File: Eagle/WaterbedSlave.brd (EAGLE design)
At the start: 55.3 x 50.4 mm, 6 parts

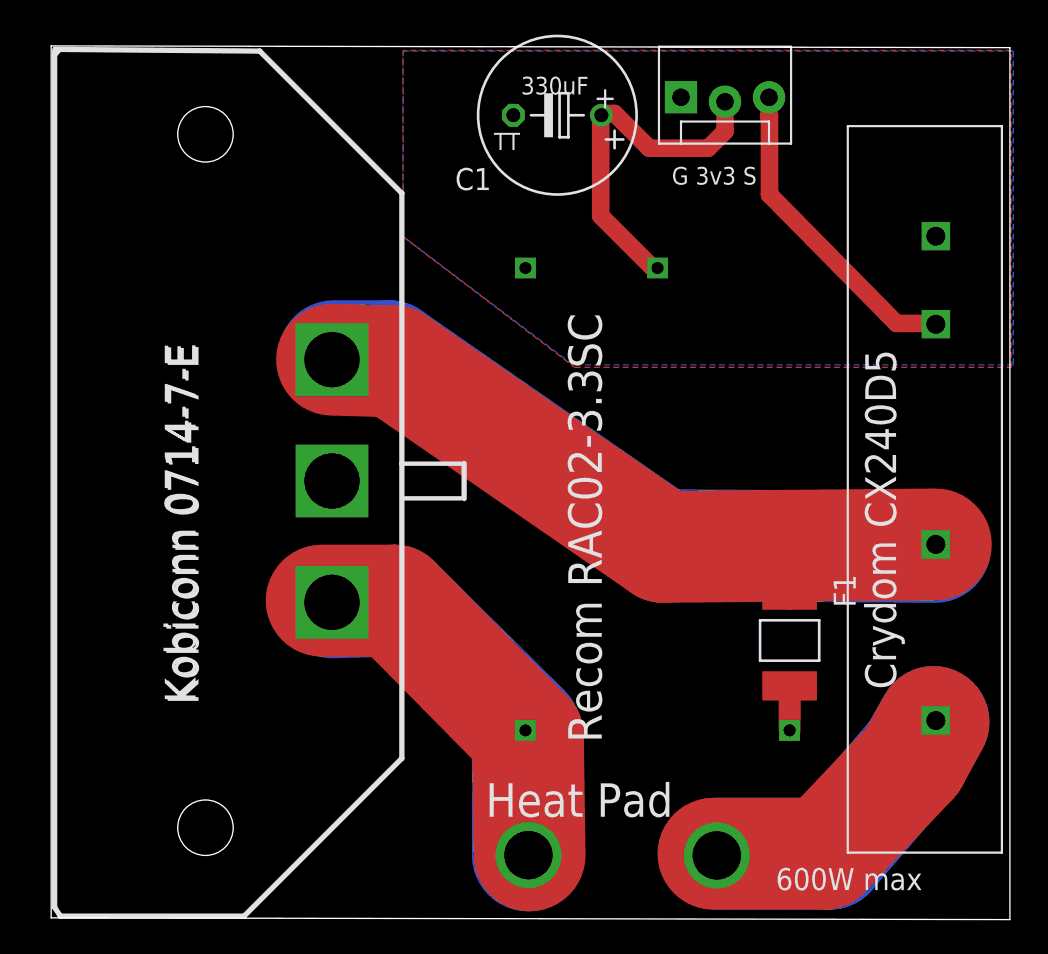
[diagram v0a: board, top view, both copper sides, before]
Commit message: Update WaterbedSlave.brd
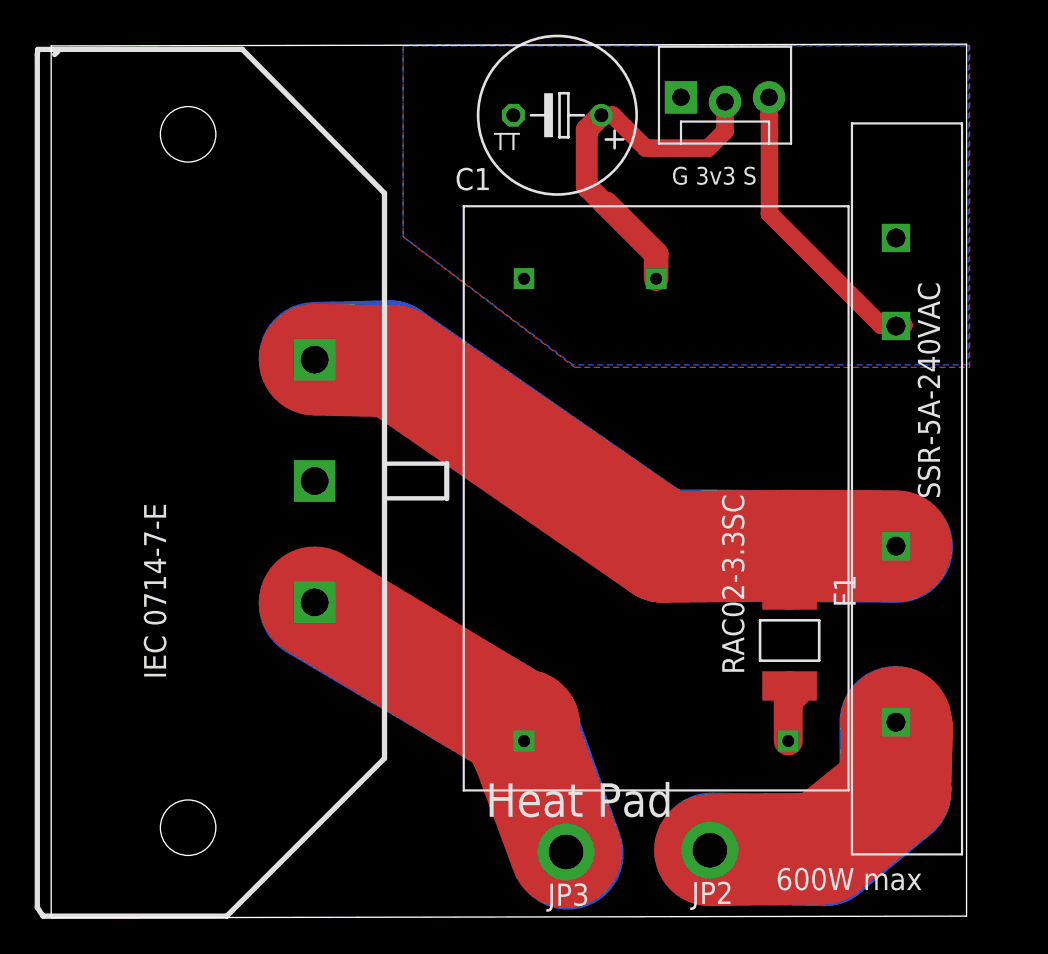
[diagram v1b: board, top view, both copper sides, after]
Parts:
- removed U$1: RAC5A240VAC, CuriousTech:RAC3V3
- added JP2, JP3: (no value), SparkFun-Connectors:1X01_2MM
- added SUPP: RAC02-3.3SC, CuriousTech:RAC02-3.3SC
- C1: value (none) -> 330uF
- U$3: value IEC -> IEC 0714-7-E
- moved U$2 2.30 mm to (48.7, 25.3)
- moved U$3 1.00 mm to (7.90, 25.2)
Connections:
- removed net G: U$3.G
- new net N$6: JP2.1, U$2.P$4
- net GND: now also SUPP.3V3; no longer U$1.P$3
- net N$1: now also JP3.1, SUPP.AC1; no longer U$1.P$1
- net N$12: now also SUPP.AC2; no longer U$1.P$2
- net N$15: now also SUPP.GND; no longer U$1.P$4
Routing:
- net N$5: track 16.3 -> 0.00 mm
- net N$11: track 16.3 -> 0.00 mm
- net N$6: track 0.00 -> 15.8 mm
- net N$3: track 6.90 -> 21.7 mm
- net N$1: track 14.2 -> 22.7 mm
- net N$4: track 22.1 -> 15.8 mm
- net N$14: track 41.0 -> 39.7 mm
- net N$2: track 38.1 -> 37.0 mm
- net N$15: track 20.5 -> 21.5 mm
- net N$12: track 2.56 -> 3.56 mm
- net N$16: track 18.5 -> 17.7 mm
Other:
- board size 55.3 x 50.4 mm -> 52.8 x 50.4 mm
- board text removed: "+"
- board text removed: "330uF"
- board text removed: "Crydom CX240D5"
- board text removed: "Kobiconn 0714-7-E"
- board text removed: "Recom RAC02-3.3SC"
